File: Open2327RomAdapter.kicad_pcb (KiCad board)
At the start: 2 copper layers, 19.6 x 43.2 mm, 7 parts, among them P1 CONN_01X04, U1 2364, U2 27128

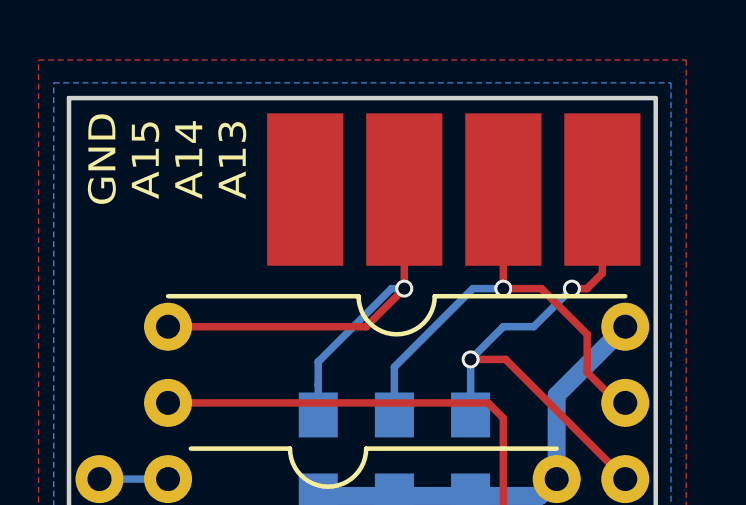
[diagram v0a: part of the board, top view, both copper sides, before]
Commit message: Update board This should be the board that went to prototype production. It has been tested and is working great!
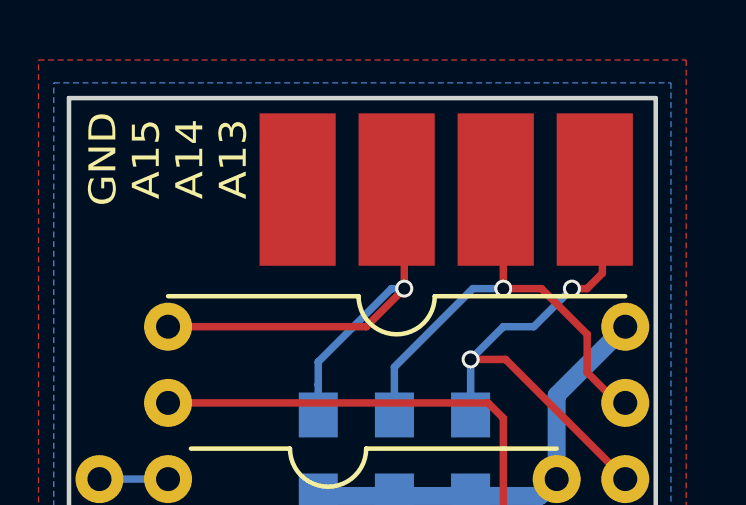
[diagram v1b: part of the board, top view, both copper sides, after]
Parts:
- U1: footprint Sukko:DIP-24_W15.24mm-Notch -> Open2327RomAdapter:DIP-24_W15.24mm-Notch
- U2: footprint Sukko:DIP-28_W15.24mm-Notch -> Open2327RomAdapter:DIP-28_W15.24mm-Notch
- turned P1 to 0 degrees
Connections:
- P1 pad 1: Net-(P1-Pad1) -> GND
- P1 pad 4: GND -> Net-(P1-Pad4)
- R1 pad 1: Net-(P1-Pad1) -> Net-(P1-Pad4)
- R2 pad 1: Net-(P1-Pad2) -> Net-(P1-Pad3)
- R3 pad 1: Net-(P1-Pad3) -> Net-(P1-Pad2)
- U2 pad 1: Net-(P1-Pad3) -> Net-(P1-Pad2)
- U2 pad 26: Net-(P1-Pad1) -> Net-(P1-Pad4)
- U2 pad 27: Net-(P1-Pad2) -> Net-(P1-Pad3)
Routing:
- net Net-(P1-Pad4): track 0.00 -> 17.0 mm, vias 0 -> 2
- net Net-(P1-Pad1): track 17.0 -> 0.00 mm, vias 2 -> 0
- net Net-(P1-Pad3): track 17.4 -> 16.0 mm
- net Net-(P1-Pad2): track 16.0 -> 17.4 mm

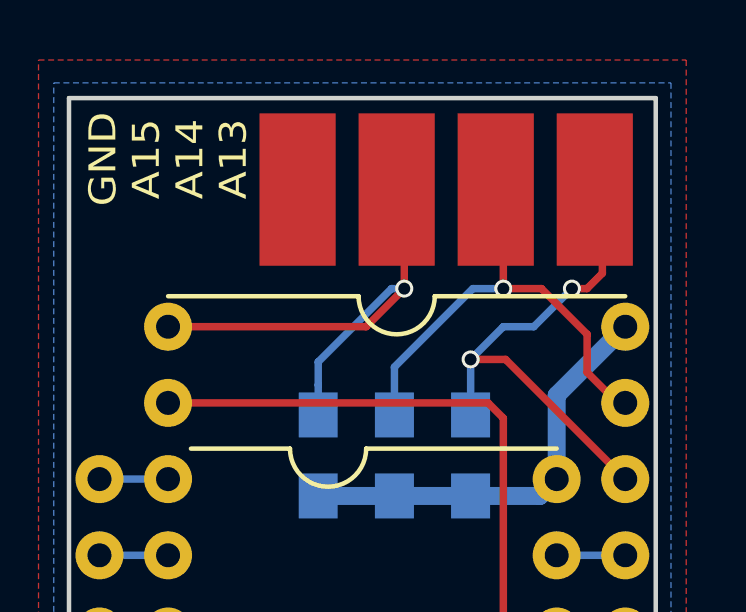
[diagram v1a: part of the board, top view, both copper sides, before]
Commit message: Cleanup
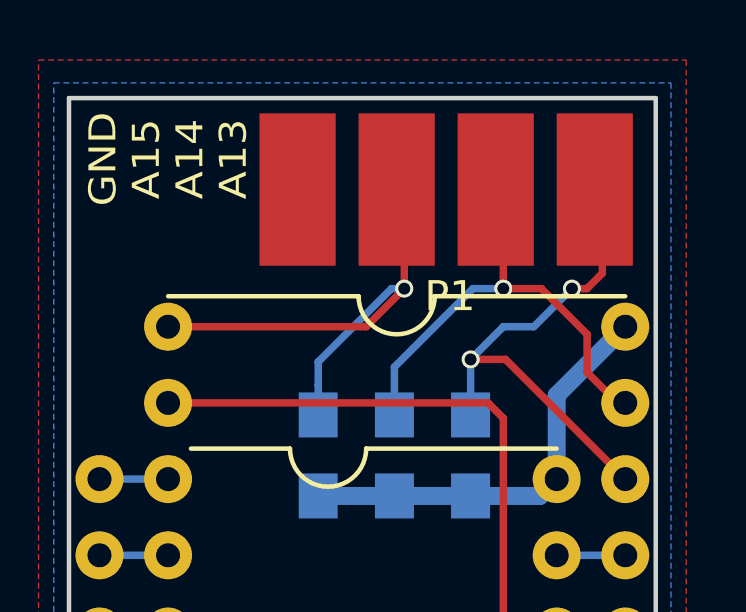
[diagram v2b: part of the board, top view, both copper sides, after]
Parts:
- P1: footprint Sukko:LoosePads-4 -> Open2327RomAdapter:LoosePads-4
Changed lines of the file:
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@@
     )
-  )
-  (module Sukko:LoosePads-4 (layer F.Cu)
-    (at 157.988 97.028)
-    (fp_text reference P1 (at 0 3.556) (layer F.SilkS) hide
-      (effects (font (size 1 1) (thickness 0.15)))
-    )
-    (fp_text value CONN_01X04 (at 0 -3.556) (layer F.Fab) hide
-      (effects (font (size 1 1) (thickness 0.15)))
-    )
-    (pad 1 smd rect (at -5.08 0 90) (size 5.08 2.54) (layers F.Cu F.Paste F.Mask)
-      (net 1 GND))
-    (pad 2 smd rect (at -1.778 0 90) (size 5.08 2.54) (layers F.Cu F.Paste F.Mask)
-      (net 25 "Net-(P1-Pad2)"))
-    (pad 3 smd rect (at 1.524 0 90) (size 5.08 2.54) (layers F.Cu F.Paste F.Mask)
-      (net 26 "Net-(P1-Pad3)"))
-    (pad 4 smd rect (at 4.826 0 90) (size 5.08 2.54) (layers F.Cu F.Paste F.Mask)
-      (net 27 "Net-(P1-Pad4)"))
   )
   (module Resistors_SMD:R_0805_HandSoldering (layer B.Cu)
@@
     )
   )
+  (module Open2327RomAdapter:LoosePads-4 (layer F.Cu)
+    (at 157.988 97.028)
+    (fp_text reference P1 (at 0 3.556) (layer F.SilkS)
+      (effects (font (size 1 1) (thickness 0.15)))
+    )
+    (fp_text value CONN_01X04 (at 0 -3.556) (layer F.Fab) hide
+      (effects (font (size 1 1) (thickness 0.15)))
+    )
+    (pad 1 smd rect (at -5.08 0 90) (size 5.08 2.54) (layers F.Cu F.Paste F.Mask)
+      (net 1 GND))
+    (pad 2 smd rect (at -1.778 0 90) (size 5.08 2.54) (layers F.Cu F.Paste F.Mask)
+      (net 25 "Net-(P1-Pad2)"))
+    (pad 3 smd rect (at 1.524 0 90) (size 5.08 2.54) (layers F.Cu F.Paste F.Mask)
+      (net 26 "Net-(P1-Pad3)"))
+    (pad 4 smd rect (at 4.826 0 90) (size 5.08 2.54) (layers F.Cu F.Paste F.Mask)
+      (net 27 "Net-(P1-Pad4)"))
+  )
   (gr_text "GND\nA15\nA14\nA13" (at 148.59 96.012 90) (layer F.SilkS)
